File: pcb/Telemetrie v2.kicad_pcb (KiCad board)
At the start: 4 copper layers, 100 x 91 mm, 78 parts, among them J1 Conn_02x03_Odd_Even, J2 Conn_01x02_Pin, J3 SMA SMD, J4 Conn_01x04_Pin, J5 Conn_01x02_Pin, M1 Conn_01x01_Pin, M2 Conn_01x01_Pin, M3 Conn_01x01_Pin, M4 Conn_01x01_Pin, U1 AVR128DB64x-xPT, U2 RC1780HP

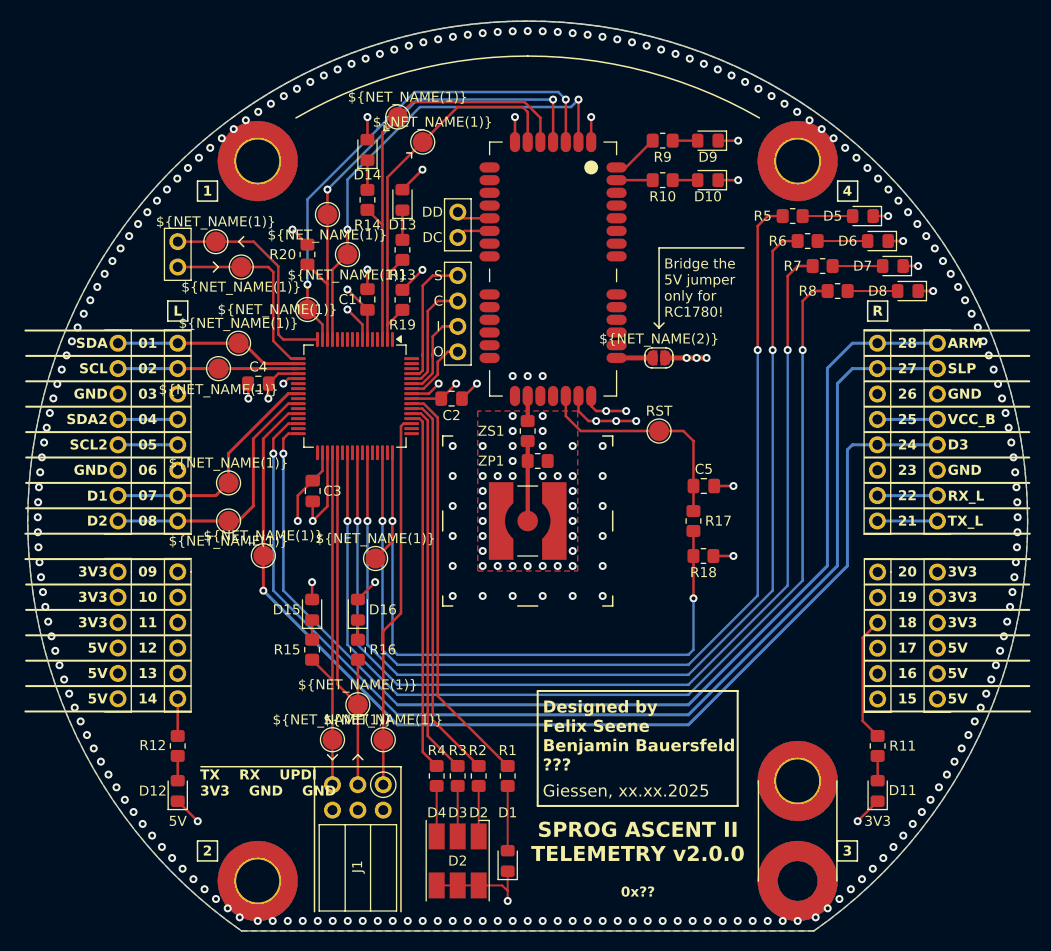
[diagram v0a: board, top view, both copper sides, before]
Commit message: pcb update
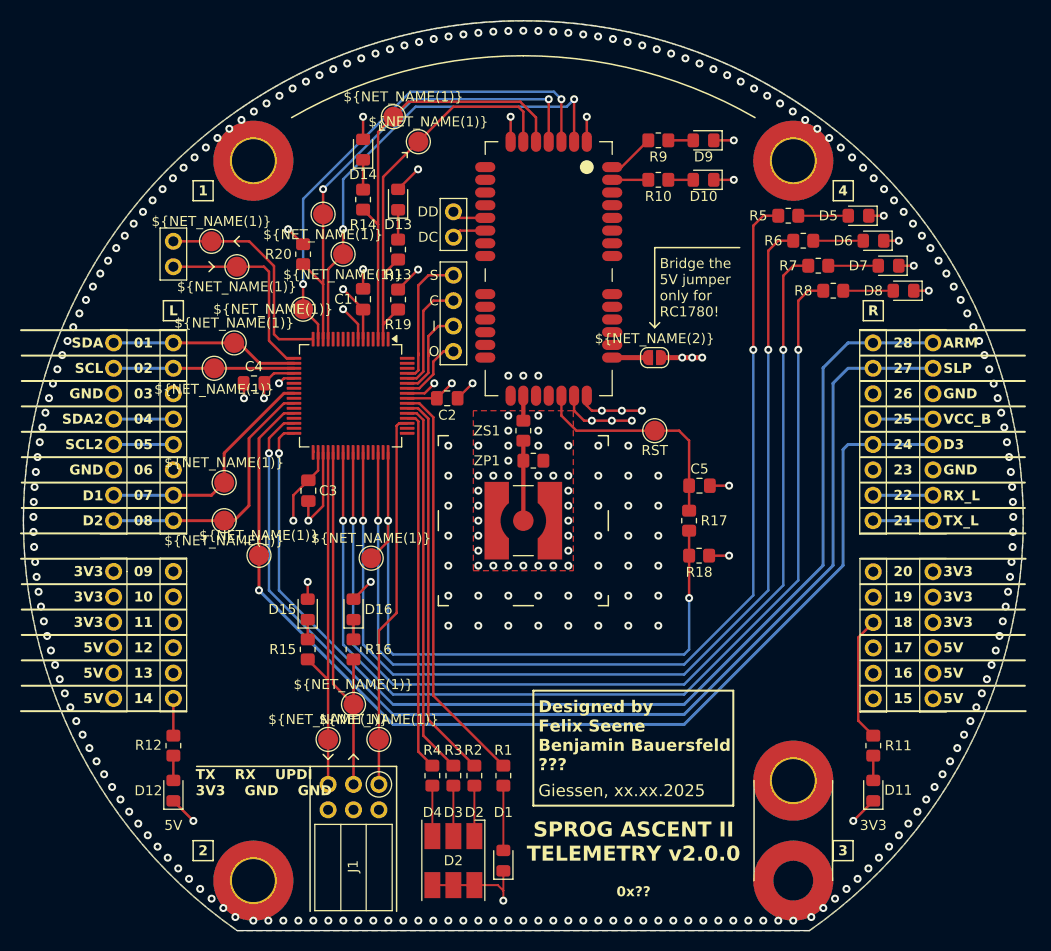
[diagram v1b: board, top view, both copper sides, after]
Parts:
- moved JR1 0.44 mm to (35.0, -17.8)
- moved JR3 0.44 mm to (41.0, -17.8)
- moved JR4 0.44 mm to (41.0, 5.10)
- moved R10 0.44 mm to (13.5, -34.1)
- moved C2 0.44 mm to (-7.61, -12.2)
- moved C3 0.44 mm to (-21.5, -3.00)
- moved C4 0.44 mm to (-26.9, -13.7)
- moved C5 0.44 mm to (17.6, -3.50)
- moved D15 0.44 mm to (-21.6, 8.87)
- moved D16 0.44 mm to (-17.0, 8.87)
- moved JP1 0.44 mm to (13.1, -16.3)
- moved R13 0.44 mm to (-12.5, -27.1)
- moved R15 0.44 mm to (-21.6, 12.9)
- moved R16 0.44 mm to (-17.0, 12.9)
- moved R19 0.44 mm to (-12.5, -22.1)
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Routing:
- net GND: track 59.1 -> 61.1 mm, vias 274 -> 294
